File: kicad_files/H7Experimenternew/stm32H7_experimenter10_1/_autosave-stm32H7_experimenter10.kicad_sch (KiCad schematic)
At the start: 79 parts, among them IC1 AD8659, IC2 78TV, IC3 AD8659, IC5 6N138, J1 SJ1-3555NG, P1 RK09SONGHUEI, P2 RK09SONGHUEI, P3 RK09SONGHUEI, P4 RK09SONGHUEI, P5 RK09SONGHUEI, P6 RK09SONGHUEI

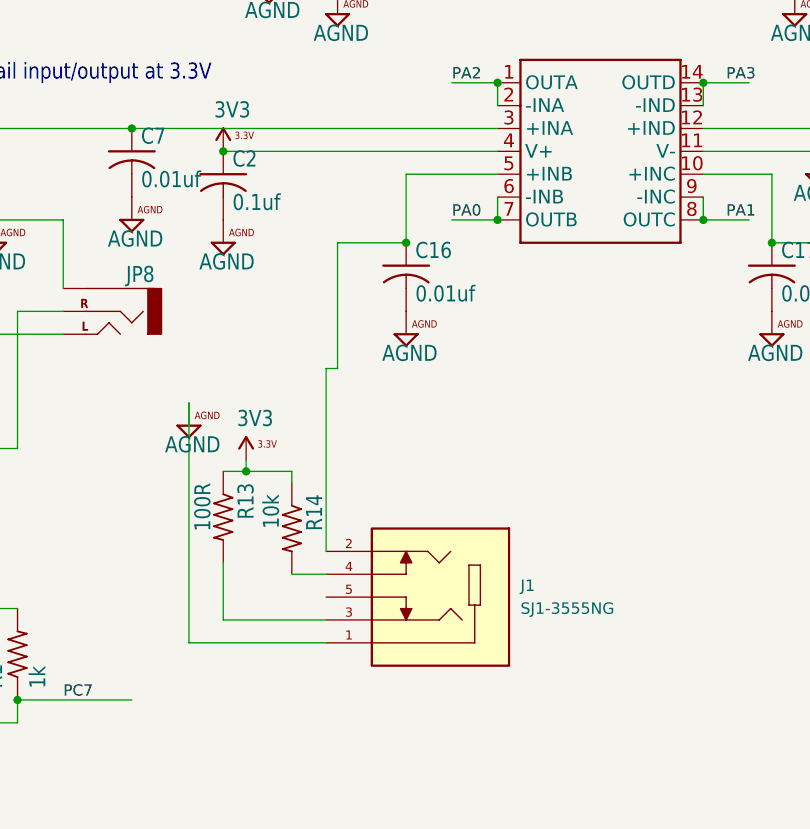
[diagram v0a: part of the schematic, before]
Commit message: new kicad
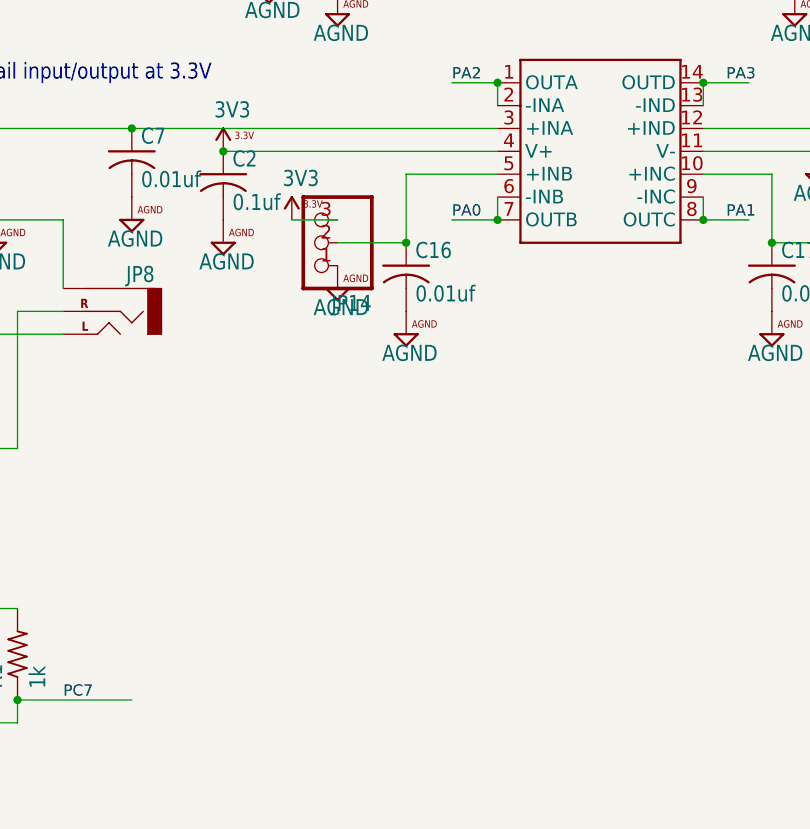
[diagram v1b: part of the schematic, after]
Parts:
- removed J1: SJ1-3555NG, Snapeda:CUI_SJ1-3555NG, symbol Snapeda:SJ1-3555NG
- removed R13: 100R, stm32H7_experimenter10:0204_5, symbol stm32H7_experimenter10-eagle-import:R-US_0204/5
- removed R14: 10k, stm32H7_experimenter10:0204_5, symbol stm32H7_experimenter10-eagle-import:R-US_0204/5
- added JP14: PINHD-1X3, stm32H7_experimenter10:1X03, symbol stm32H7_experimenter10-eagle-import:PINHD-1X3
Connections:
- net 3V3: now also JP14.3
- net AGND: now also JP14.1
- net at C16.1, IC3.5 (+INB): now also JP14.2
